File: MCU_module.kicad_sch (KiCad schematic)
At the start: 7 parts, among them U1 STM32C011F4U6TR, Y1 Crystal

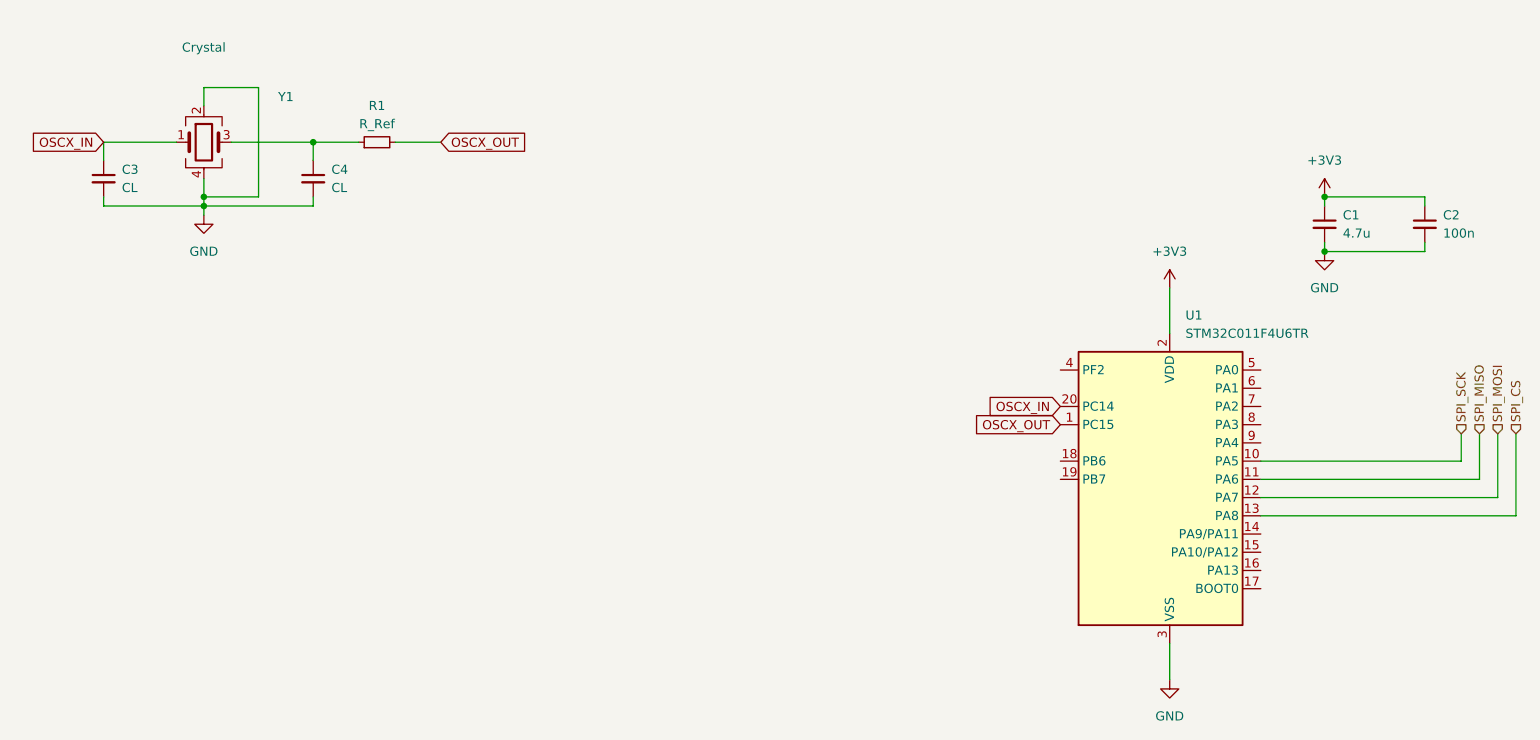
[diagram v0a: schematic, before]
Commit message: First basic design
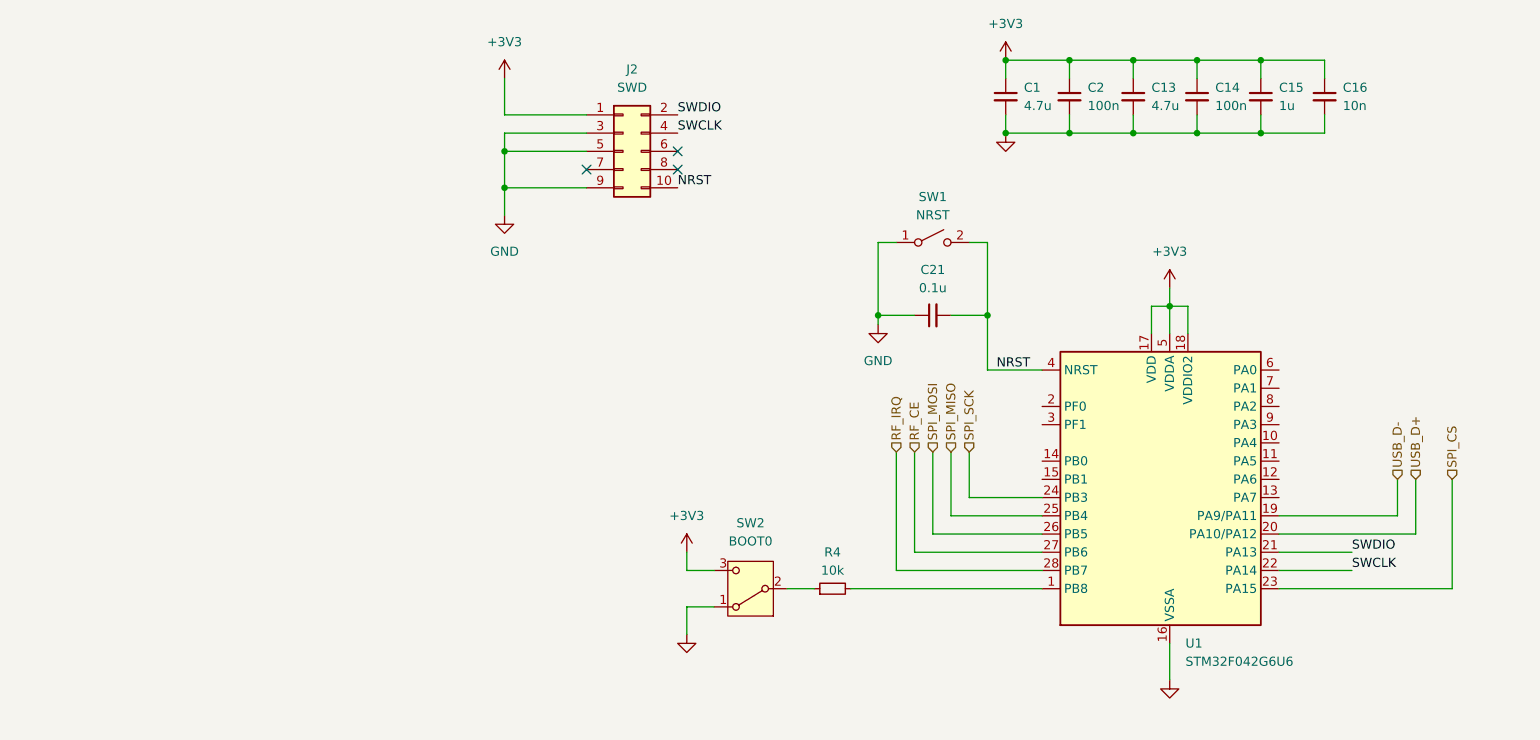
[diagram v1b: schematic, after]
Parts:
- removed C3, C4: CL, symbol Device:C_Small
- removed R1: R_Ref, symbol Device:R_Small
- removed U1: STM32C011F4U6TR, Package_DFN_QFN:ST_UFQFPN-20_3x3mm_P0.5mm, symbol MCU_ST_STM32C0:STM32C011F_4-6_Ux
- removed Y1: Crystal, symbol Device:Crystal_GND24
- added BOOT0: SW2, symbol Switch:SW_SPDT
- added C13: 4.7u, Capacitor_SMD:C_0402_1005Metric, symbol Device:C_Small
- added C14: 100n, Capacitor_SMD:C_0402_1005Metric, symbol Device:C_Small
- added C15: 1u, Capacitor_SMD:C_0402_1005Metric, symbol Device:C_Small
- added C16: 10n, Capacitor_SMD:C_0402_1005Metric, symbol Device:C_Small
- added C21: 0.1u, Capacitor_SMD:C_0402_1005Metric, symbol Device:C_Small
- added J2: SWD, Connector_PinHeader_1.27mm:PinHeader_2x05_P1.27mm_Vertical_SMD, symbol Connector_Generic:Conn_02x05_Odd_Even
- added R4: 10k, Resistor_SMD:R_0603_1608Metric, symbol Device:R_Small
- added SW1: NRST, symbol Switch:SW_SPST
- added U1: STM32F042G6U6, Package_DFN_QFN:QFN-28_4x4mm_P0.5mm, symbol MCU_ST_STM32F0:STM32F042G6Ux
- C1, C2: footprint (none) -> Capacitor_SMD:C_0402_1005Metric
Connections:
- net +3V3: now also BOOT0.3 (C), C13.1, C14.1, C15.1, C16.1, J2.1 (Pin_1), U1.17 (VDD), U1.18 (VDDIO2), U1.5 (VDDA)
- net GND: now also BOOT0.1 (A), C13.2, C14.2, C15.2, C16.2, C21.1, J2.3 (Pin_3), J2.5 (Pin_5), J2.9 (Pin_9), SW1.1 (A), U1.16 (VSSA)
- net SPI_CS: now also U1.23 (PA15)
- net SPI_MISO: now also U1.25 (PB4)
- net SPI_MOSI: now also U1.26 (PB5)
- net SPI_SCK: now also U1.24 (PB3)
- new net: BOOT0.2 (B), R4.1
- new net: R4.2, U1.1 (PB8)
- new net NRST: C21.2, J2.10 (Pin_10), SW1.2 (B), U1.4 (NRST)
- new net RF_CE: U1.27 (PB6)
- new net RF_IRQ: U1.28 (PB7)
- new net SWCLK: J2.4 (Pin_4), U1.22 (PA14)
- new net SWDIO: J2.2 (Pin_2), U1.21 (PA13)
- new net USB_D+: U1.20 (PA10/PA12)
- new net USB_D-: U1.19 (PA9/PA11)
- no-connect marks 0 -> 3
